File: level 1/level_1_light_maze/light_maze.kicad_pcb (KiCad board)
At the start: 2 copper layers, 88 x 33 mm, 35 parts, among them J1 Conn_01x02_Socket, J2 Conn_01x03_Socket, J3 Conn_01x03_Socket, J4 Conn_01x03_Socket, J5 Conn_01x03_Socket, J6 Conn_01x03_Socket, J7 Conn_01x03_Socket, J8 Conn_01x03_Socket, J9 Conn_01x03_Socket, U2 LM339

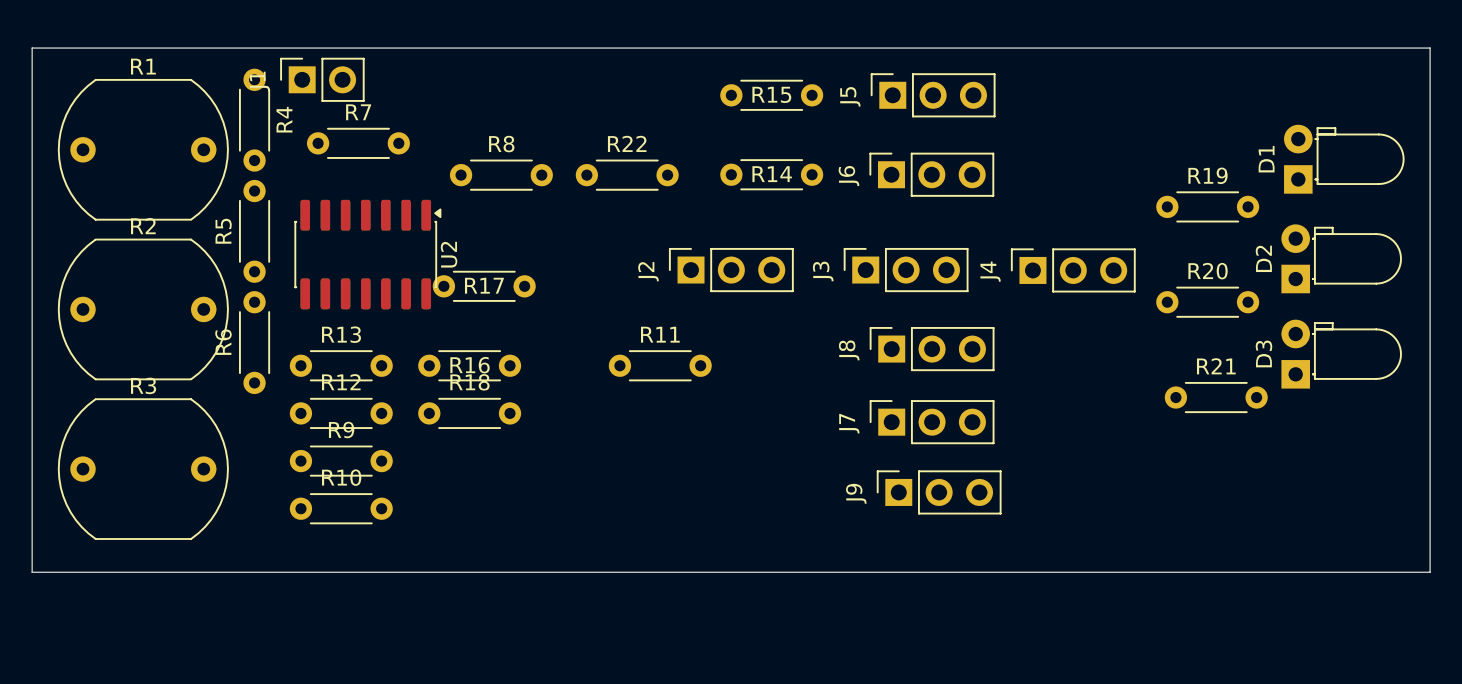
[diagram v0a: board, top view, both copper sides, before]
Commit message: pcb update
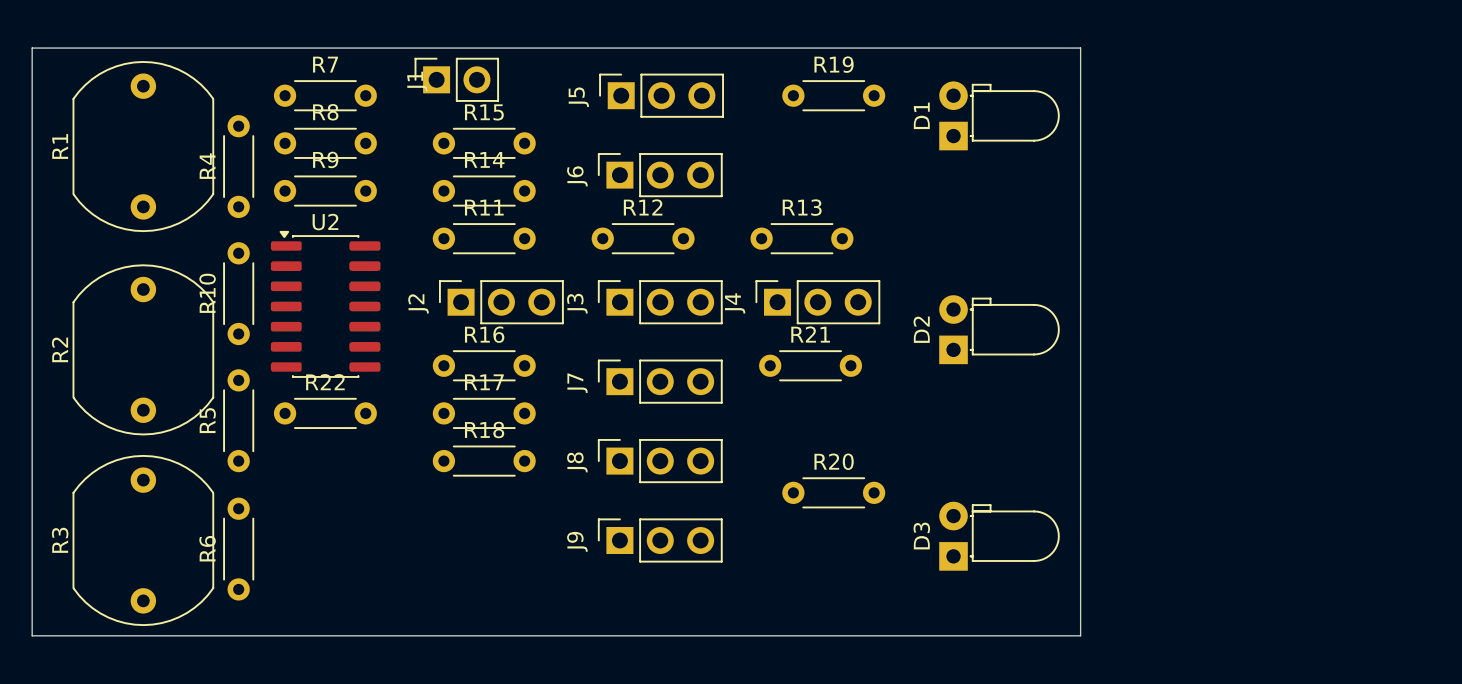
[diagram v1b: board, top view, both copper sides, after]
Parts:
- moved R13 30.1 mm to (159.9, 105.0)
- moved R20 26.4 mm to (161.9, 121.0)
- moved R21 25.6 mm to (160.5, 113.0)
- moved R19 24.6 mm to (161.9, 96.0)
- moved D3 24.4 mm to (172.0, 125.0)
- moved R22 24.2 mm to (129.9, 116.0)
- moved D2 22.0 mm to (172.0, 112.0)
- moved R12 22.0 mm to (149.9, 105.0)
- moved D1 21.9 mm to (172.0, 98.5)
- moved J8 18.5 mm to (151.0, 119.0)
- moved R15 18.3 mm to (139.9, 99.0)
- moved R14 18.1 mm to (139.9, 102.0)
- moved J9 17.8 mm to (151.0, 124.0)
- moved J7 17.3 mm to (151.0, 114.0)
- moved J5 17.1 mm to (151.1, 96.0)
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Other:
- board size 88 x 33 mm -> 66 x 37 mm

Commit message: light_maze_pcb_edit
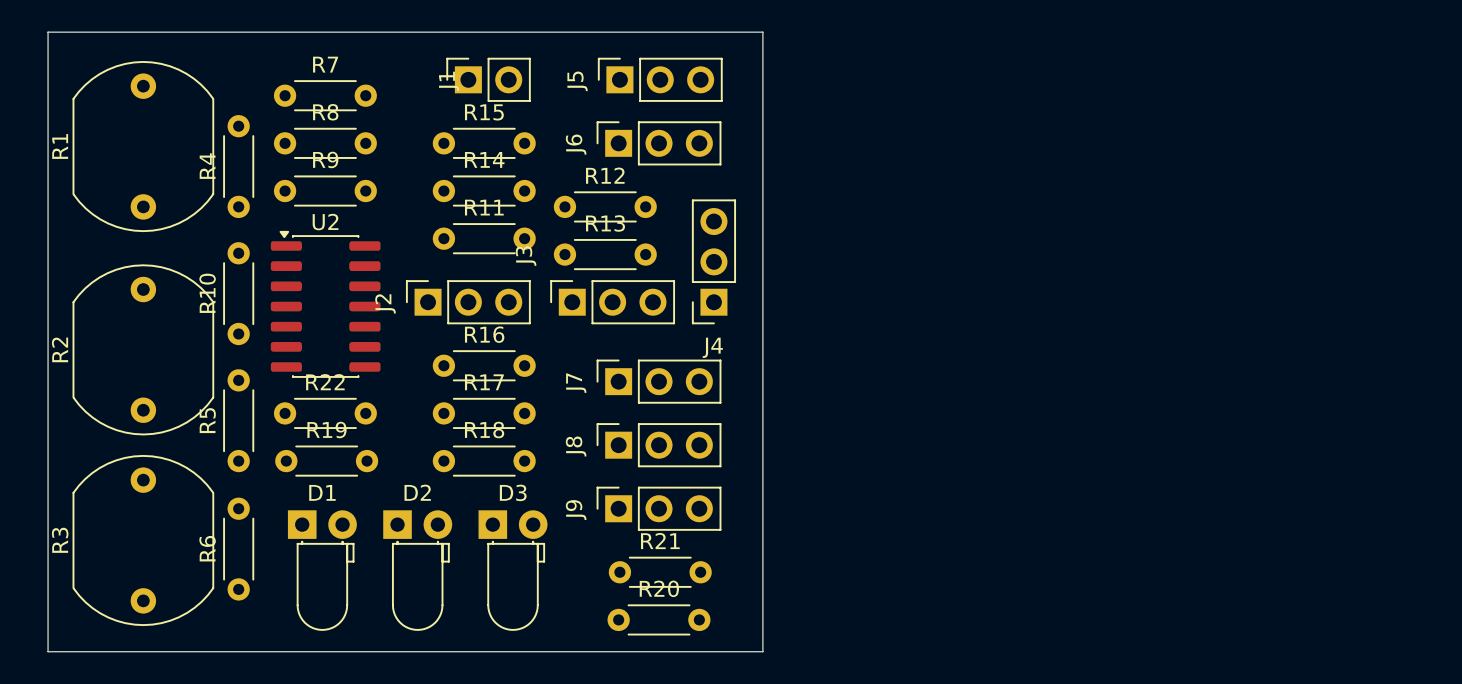
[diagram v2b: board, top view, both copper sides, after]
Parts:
- moved D1 47.7 mm to (131.0, 123.0), turned to 0 degrees
- moved R19 39.3 mm to (130.0, 119.0)
- moved D2 36.7 mm to (137.0, 123.0), turned to 0 degrees
- moved D3 29.1 mm to (143.0, 123.0), turned to 0 degrees
- moved R21 16.1 mm to (151.0, 126.0)
- moved R20 13.6 mm to (150.9, 129.0)
- moved R13 12.4 mm to (147.5, 106.0)
- moved J4 4.00 mm to (156.9, 109.0), turned to 180 degrees
- moved R12 3.11 mm to (147.5, 103.0)
- moved J3 3.00 mm to (148.0, 109.0)
- moved J2 2.08 mm to (138.9, 109.0)
- moved J6 2.00 mm to (150.9, 99.0)
- moved J9 2.00 mm to (150.9, 122.0)
- moved J1 2.00 mm to (141.5, 95.0)
- moved J5 1.00 mm to (151.0, 95.0)
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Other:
- board size 66 x 37 mm -> 45 x 39 mm
